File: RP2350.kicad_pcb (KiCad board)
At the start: 2 copper layers, 37.7 x 47.5 mm, 48 parts, among them J1 SM03B-SRSS-TB, J3 FC68145S, J5 SM04B-GHS-TB_LF__SN_-, J7 SM06B-GHS-TB, J9 USB_C_Receptacle_USB2.0_16P, U2 RP2350_60QFN, U3 NCP1117-3.3_SOT223, U4 W25Q128JVPIQ TR, X2 ABM8-272-T3

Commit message: Comment and edit gitignore
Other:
- board text added: "Match board edges with connectors, check with 3d models"
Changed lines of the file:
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@@
 		(layer "Edge.Cuts")
+	)
+	(gr_text "Match board edges with connectors,\ncheck with 3d models"
+		(at 164 93 0)
+		(layer "Cmts.User")
+		(effects
+			(font
+				(size 1 1)
+				(thickness 0.15)
+			)
+			(justify left bottom)
+		)
 	)
 	(dimension

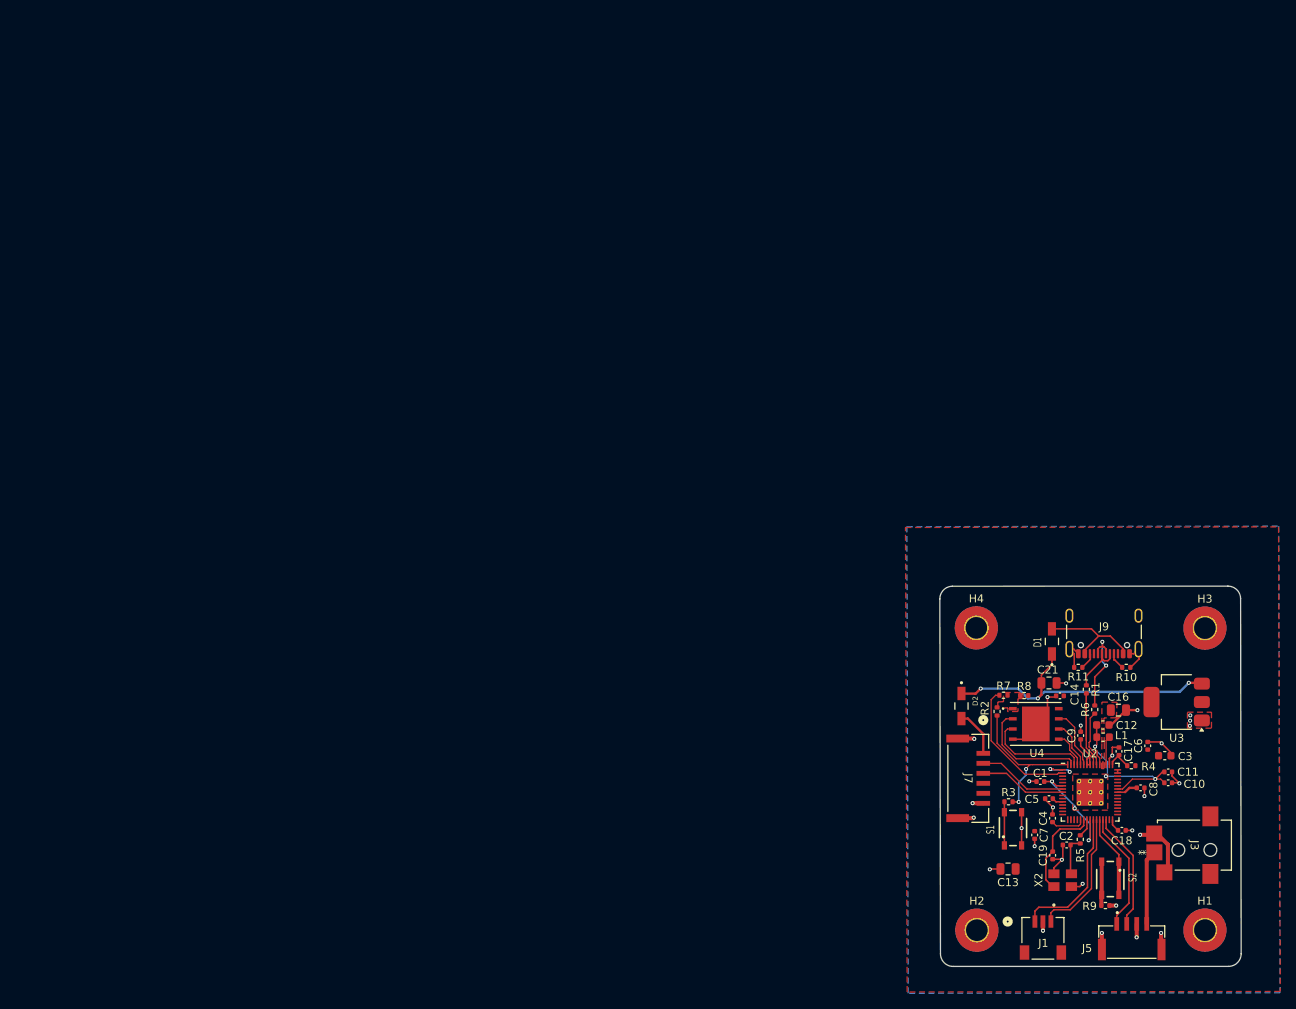
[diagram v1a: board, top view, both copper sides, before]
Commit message: edge edits
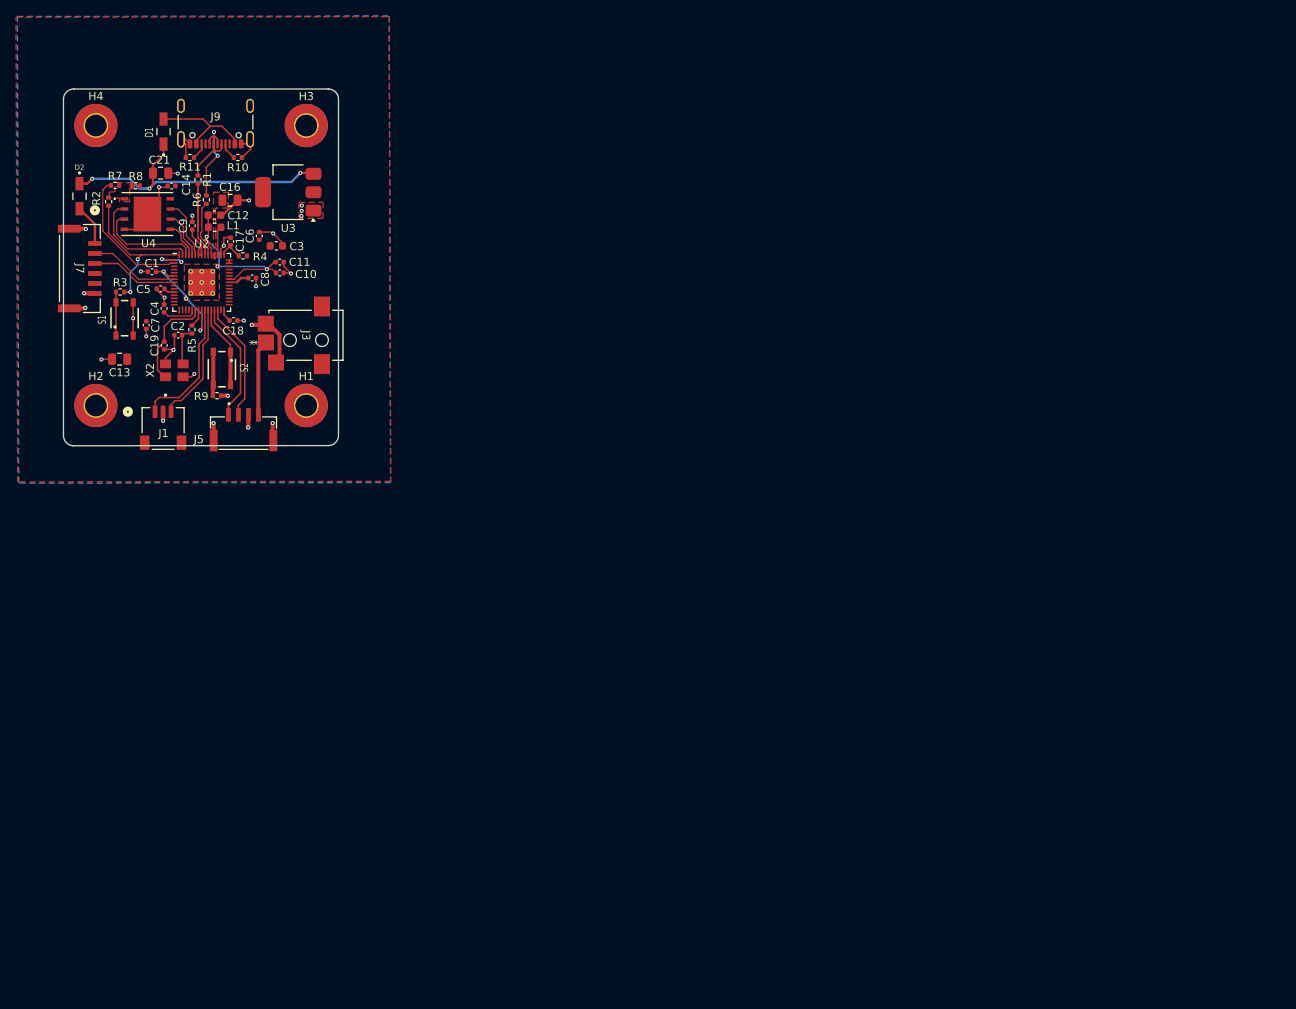
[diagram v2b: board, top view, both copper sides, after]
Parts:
- moved H1 130.1 mm to (79.2, 76.2)
- moved H3 128.7 mm to (79.2, 41.2)
- moved H2 128.2 mm to (52.9, 76.2)
- moved C13 128.0 mm to (55.8, 70.4)
- moved C14 128.0 mm to (62.3, 48.7)
- moved C17 128.0 mm to (69.7, 55.7)
- moved C21 128.0 mm to (60.9, 47.1)
- moved C3 128.0 mm to (75.4, 56.2)
- moved C4 128.0 mm to (61.4, 64.0)
- moved C5 128.0 mm to (60.9, 61.6)
- moved C6 128.0 mm to (73.3, 55.0)
- moved J7 128.0 mm to (50.9, 59.0)
- moved R10 128.0 mm to (70.6, 45.2)
- moved R11 128.0 mm to (64.6, 45.2)
- moved R5 128.0 mm to (64.8, 66.7)
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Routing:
- net /SWD: track 17.0 -> 15.1 mm
- net /SWCLK: track 17.9 -> 16.8 mm
- net VBUS: track 37.9 -> 37.1 mm
- net /VCC_5V: track 5.94 -> 5.14 mm
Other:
- board size 37.7 x 47.5 mm -> 34.4 x 44.6 mm
